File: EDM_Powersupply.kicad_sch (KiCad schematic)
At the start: 23 parts, among them J1 Screw_Terminal_01x02, Q1 IPW65R037C6, U1 L7805, U2 STGAP2SM, U3 RP2040, U4 MGJ2D051505SC, U5 LMV331

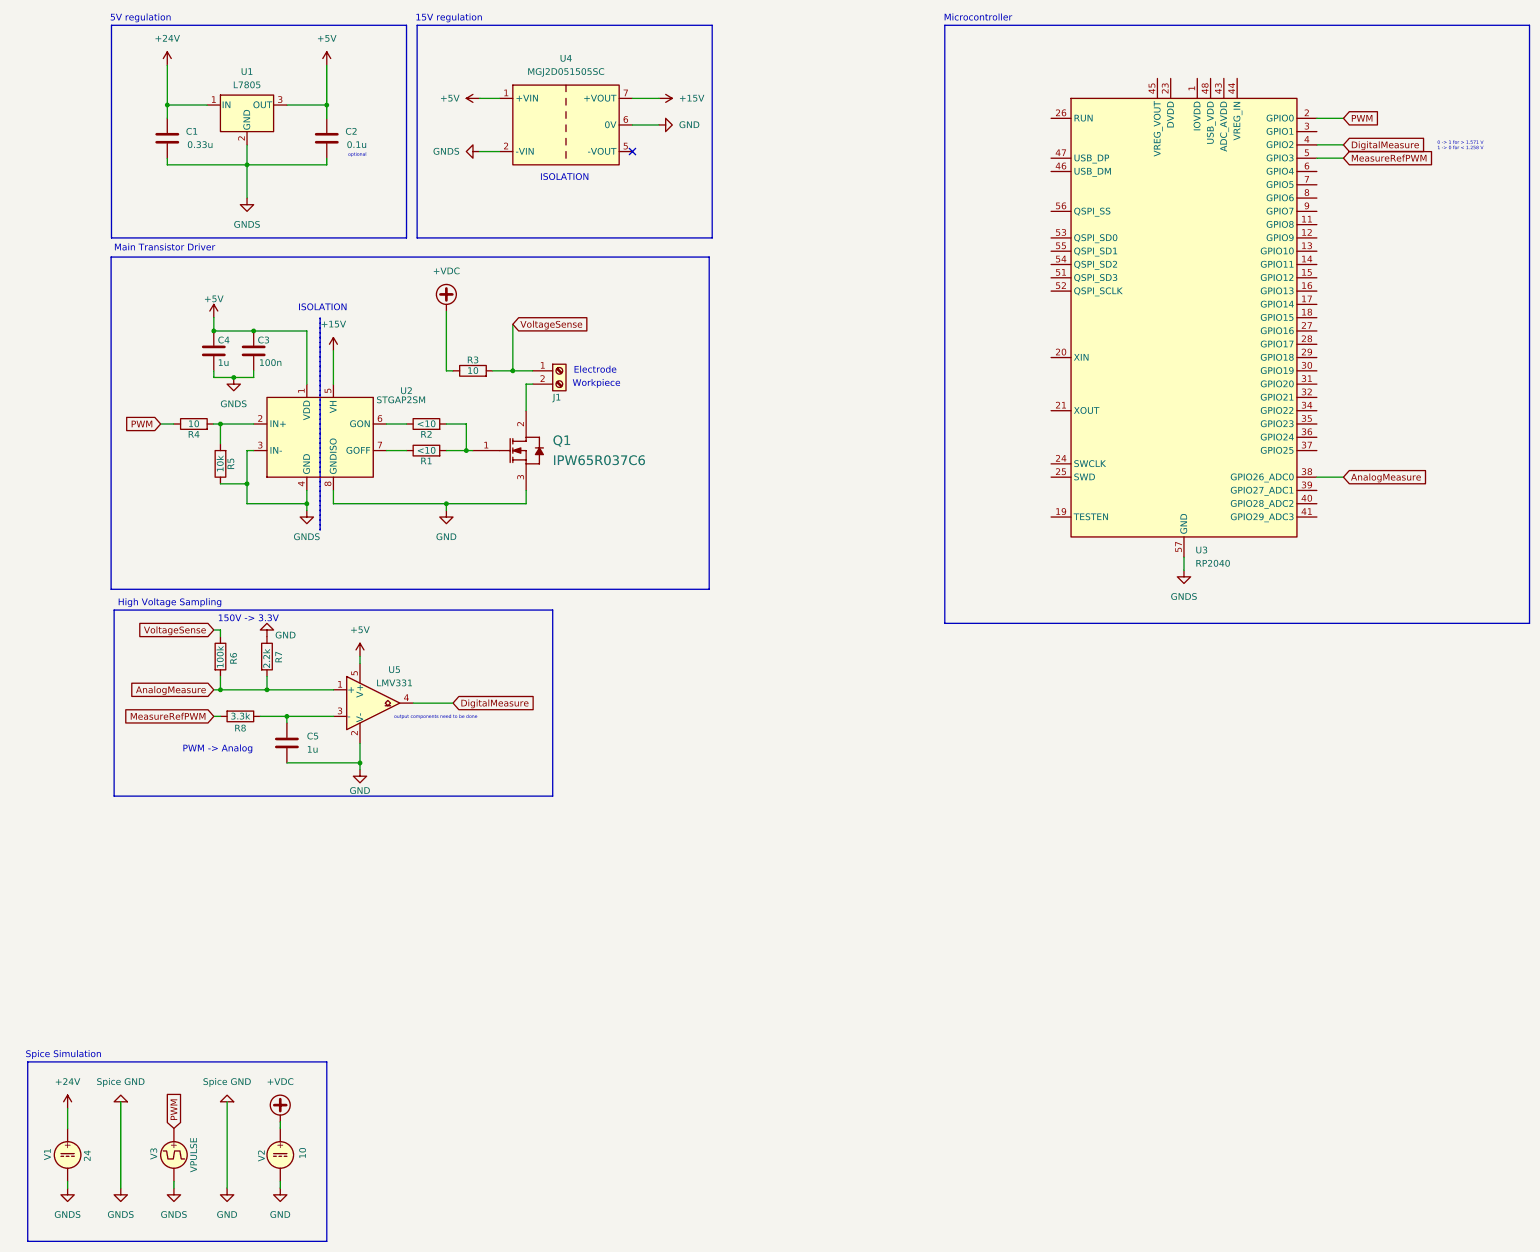
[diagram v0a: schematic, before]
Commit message: Signal isolation concept
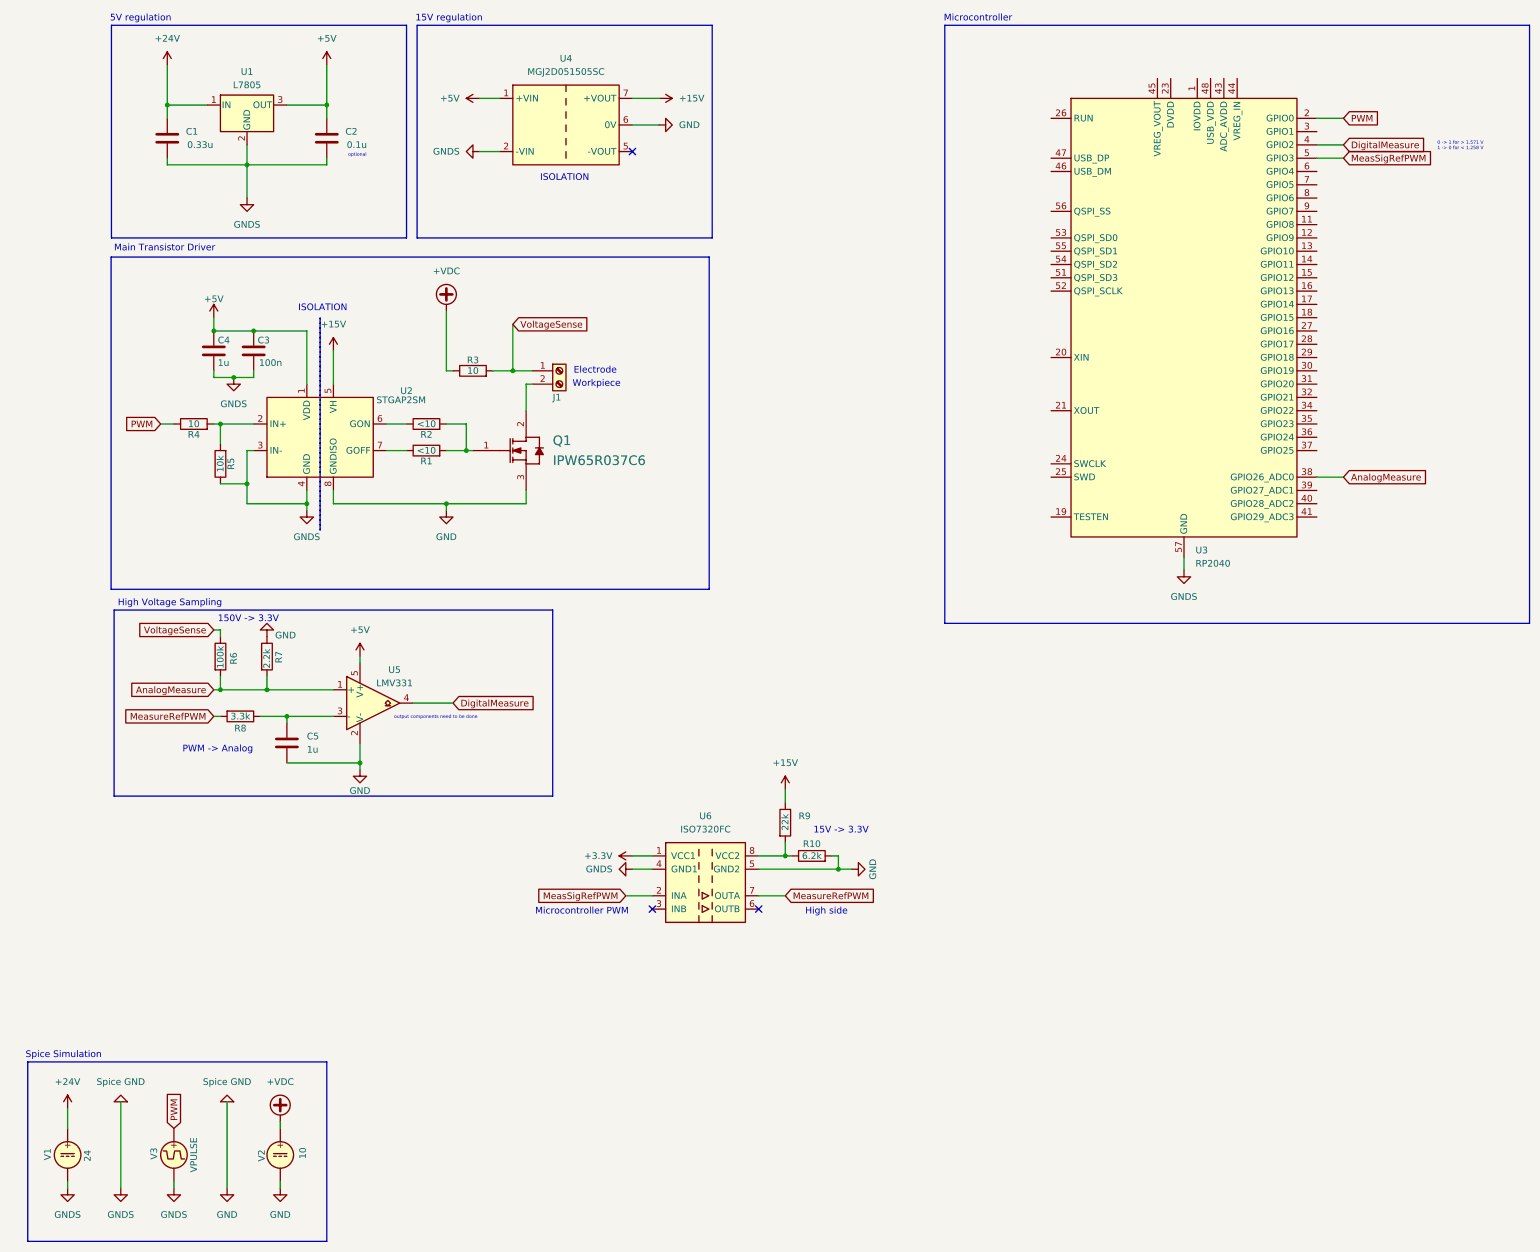
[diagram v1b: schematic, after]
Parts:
- added R10: 6.2k, symbol Device:R
- added R9: 22k, symbol Device:R
- added U6: ISO7320FC, Package_SO:SOIC-8_3.9x4.9mm_P1.27mm, symbol Isolator:ISO7320FC
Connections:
- net +15V: now also R9.1
- net GND: now also R10.2, U6.4 (GND1), U6.5 (GND2)
- net MeasureRefPWM: now also U6.7 (OUTA); no longer U3.5 (GPIO3)
- new net: R10.1, R9.2, U6.8 (VCC2)
- new net +3.3V: U6.1 (VCC1)
- new net MeasSigRefPWM: U3.5 (GPIO3), U6.2 (INA)
- no-connect marks 1 -> 3
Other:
- note added: "15V -> 3.3V"
- note added: "High side"
- note added: "Microcontroller PWM"
